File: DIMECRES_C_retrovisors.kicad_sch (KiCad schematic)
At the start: 65 parts, among them J10 Vbat, J2 DE9_Pins, J3 Conn_01x05_Pin, J4 Motor3, J6 Intermitente, J7 Calentador, J8 Motor2, J9 Motor1, Q1 DTC144E, Q2 DTC144E, Q3 DTC144E, SW1 SW_DPDT_G6S, U2 LM1117DT-ADJ, U3 LM2596S-ADJ, U4 L298N, U5 TJA1042T, U6 ADA4511-2, U7 PIC18F4480-IP, Y1 Crystal

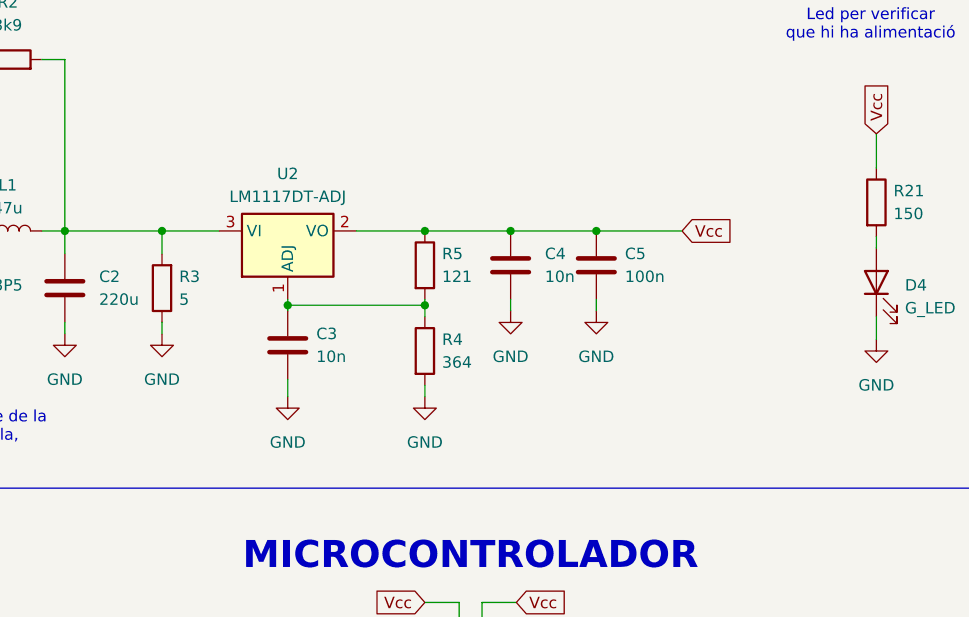
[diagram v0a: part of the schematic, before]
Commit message: Update DIMECRES_C_retrovisors.kicad_sch
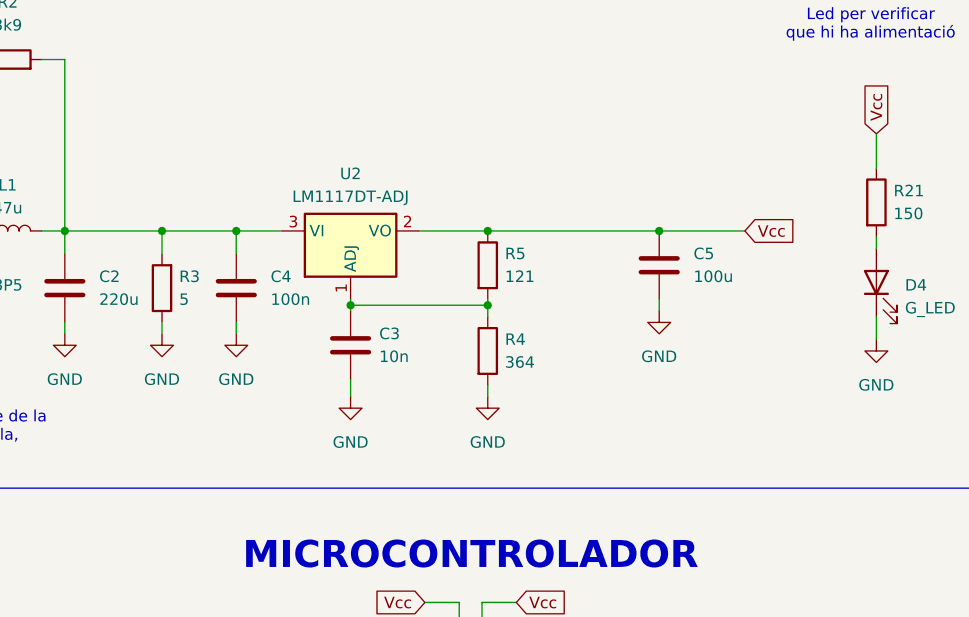
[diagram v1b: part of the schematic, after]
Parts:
- C4: value 10n -> 100n
- C5: value 100n -> 100u
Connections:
- net Vcc: no longer C4.1
- net at C2.1, L1.2, R2.2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: now also C4.1
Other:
- moved on the sheet: C3, C4, C5, R4, R5, U2
